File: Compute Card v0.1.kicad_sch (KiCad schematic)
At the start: 12 parts, among them J1 Bus_PCI_Express_x1, U1 PI7C9X440SLBFDE, U2 TPS62130A

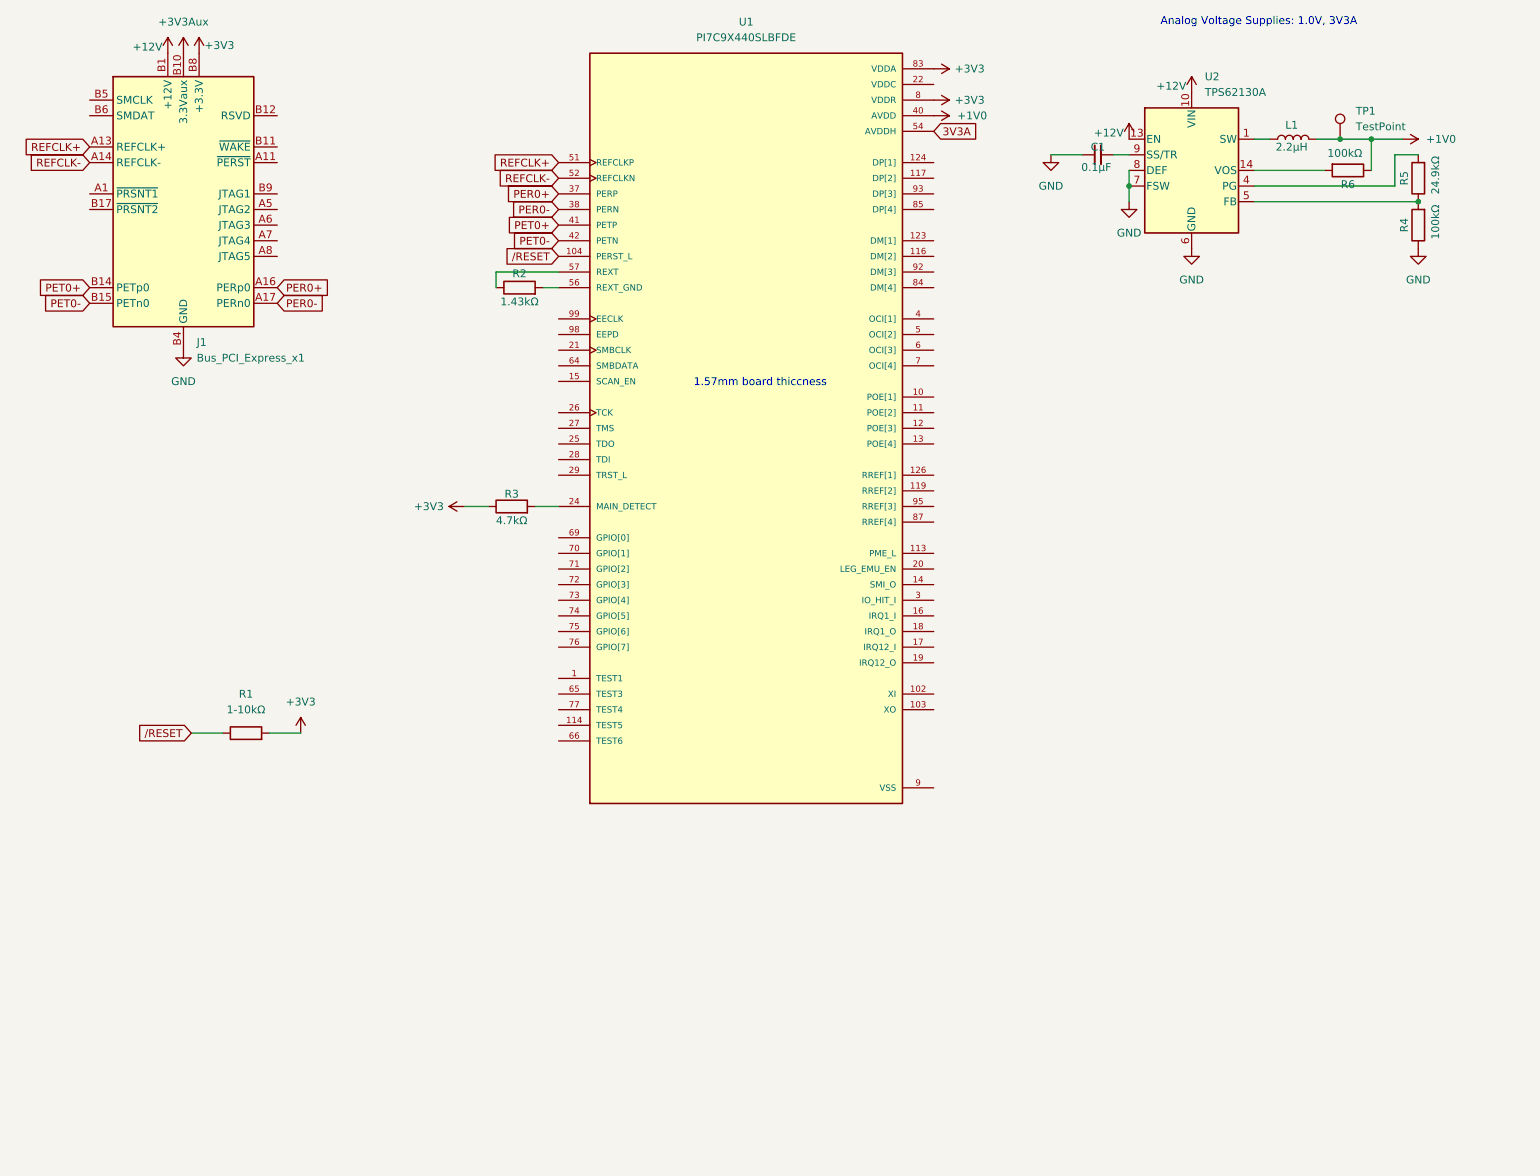
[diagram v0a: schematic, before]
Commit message: Almost Completed PCIe Interface
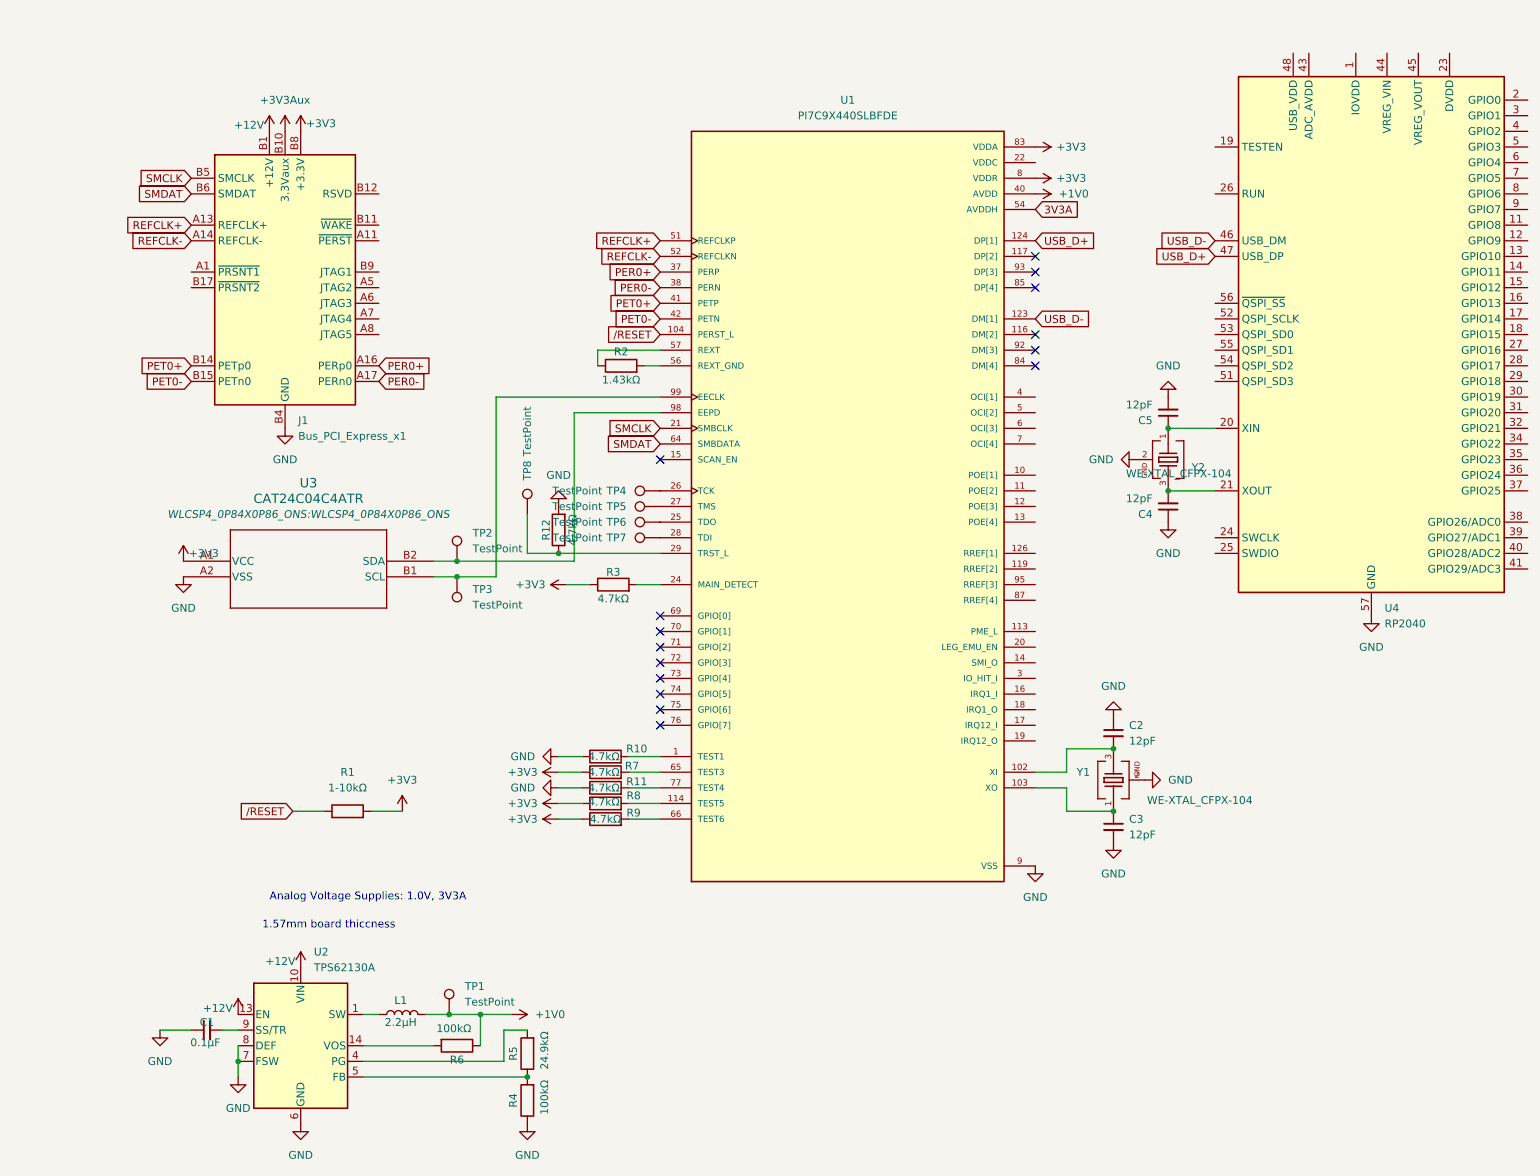
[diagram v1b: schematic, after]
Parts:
- added C2, C3, C4, C5: 12pF, Capacitor_SMD:C_0603_1608Metric, symbol Device:C_Small
- added R10, R11, R12, R7, R8, R9: 4.7kΩ, Resistor_SMD:R_0805_2012Metric_Pad1.20x1.40mm_HandSolder, symbol Device:R
- added TP2, TP3, TP4, TP5, TP6, TP7, TP8: TestPoint, TestPoint:TestPoint_Pad_D1.0mm, symbol Connector:TestPoint
- added U3: CAT24C04C4ATR, WLCSP4_0P84X0P86_ONS:WLCSP4_0P84X0P86_ONS, symbol 2026-02-08_09-35-42:CAT24C04C4ATR
- added U4: RP2040, Package_DFN_QFN:QFN-56-1EP_7x7mm_P0.4mm_EP3.2x3.2mm_ThermalVias, symbol MCU_RaspberryPi:RP2040
- added Y1, Y2: WE-XTAL_CFPX-104, WE-XTAL_CFPX-104:WE-XTAL_CFPX-104, symbol WE-XTAL_CFPX-104:WE-XTAL_CFPX-104
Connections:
- net VSS is gone; now on net GND: U1.101 (VSS), U1.106 (VSS), U1.110 (VSS), U1.118 (VSS), U1.120 (VSS), U1.125 (VSS), U1.127 (VSS), U1.129 (VSS), U1.23 (VSS), U1.34 (VSS), U1.36 (VSS), U1.39 (VSS), U1.45 (VSS), U1.50 (VSS), U1.53 (VSS), U1.61 (VSS), U1.68 (VSS), U1.82 (VSS), U1.86 (VSS), U1.89 (VSS), U1.9 (VSS), U1.94 (VSS), U1.96 (VSS)
- net +3V3: now also R7.1, R8.1, R9.1, U3.A1 (VCC)
- net GND: now also C2.1, C3.2, C4.1, C5.2, R10.1, R11.1, R12.2, U3.A2 (VSS), U4.57 (GND), Y1.2, Y1.4, Y2.2, Y2.4
- net at U1.1 (TEST1): now also R10.2
- net at U1.102 (XI): now also C2.2, Y1.3
- net at U1.103 (XO): now also C3.1, Y1.1
- net at U1.114 (TEST5): now also R8.2
- net USB_D-: now reaches U1.123 (DM[1])
- net USB_D-: now also U4.46 (USB_DM)
- net USB_D+: now reaches U1.124 (DP[1])
- net USB_D+: now also U4.47 (USB_DP)
- net SMCLK: now reaches U1.21 (SMBCLK)
- net SMCLK: now also J1.B5 (SMCLK)
- net at U1.25 (TDO): now also TP6.1
- net at U1.26 (TCK): now also TP4.1
- net at U1.27 (TMS): now also TP5.1
- net at U1.28 (TDI): now also TP7.1
- net at U1.29 (TRST_L): now also R12.1, TP8.1
- net SMDAT: now reaches U1.64 (SMBDATA)
- net SMDAT: now also J1.B6 (SMDAT)
- net at U1.65 (TEST3): now also R7.2
- net at U1.66 (TEST6): now also R9.2
- net at U1.77 (TEST4): now also R11.2
- net at U1.98 (EEPD): now also TP2.1, U3.B2 (SDA)
- net at U1.99 (EECLK): now also TP3.1, U3.B1 (SCL)
- new net: U4.1 (IOVDD), U4.10 (IOVDD), U4.22 (IOVDD), U4.33 (IOVDD), U4.42 (IOVDD), U4.49 (IOVDD)
- new net: C5.1, U4.20 (XIN), Y2.1
- new net: C4.2, U4.21 (XOUT), Y2.3
- new net: U4.23 (DVDD), U4.50 (DVDD)
- no-connect marks 0 -> 15
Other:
- moved on the sheet: C1, J1, L1, R1, R2, R3, R4, R5, R6, TP1, U1, U2
